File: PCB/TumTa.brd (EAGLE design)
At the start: 100 x 80 mm, 20 parts

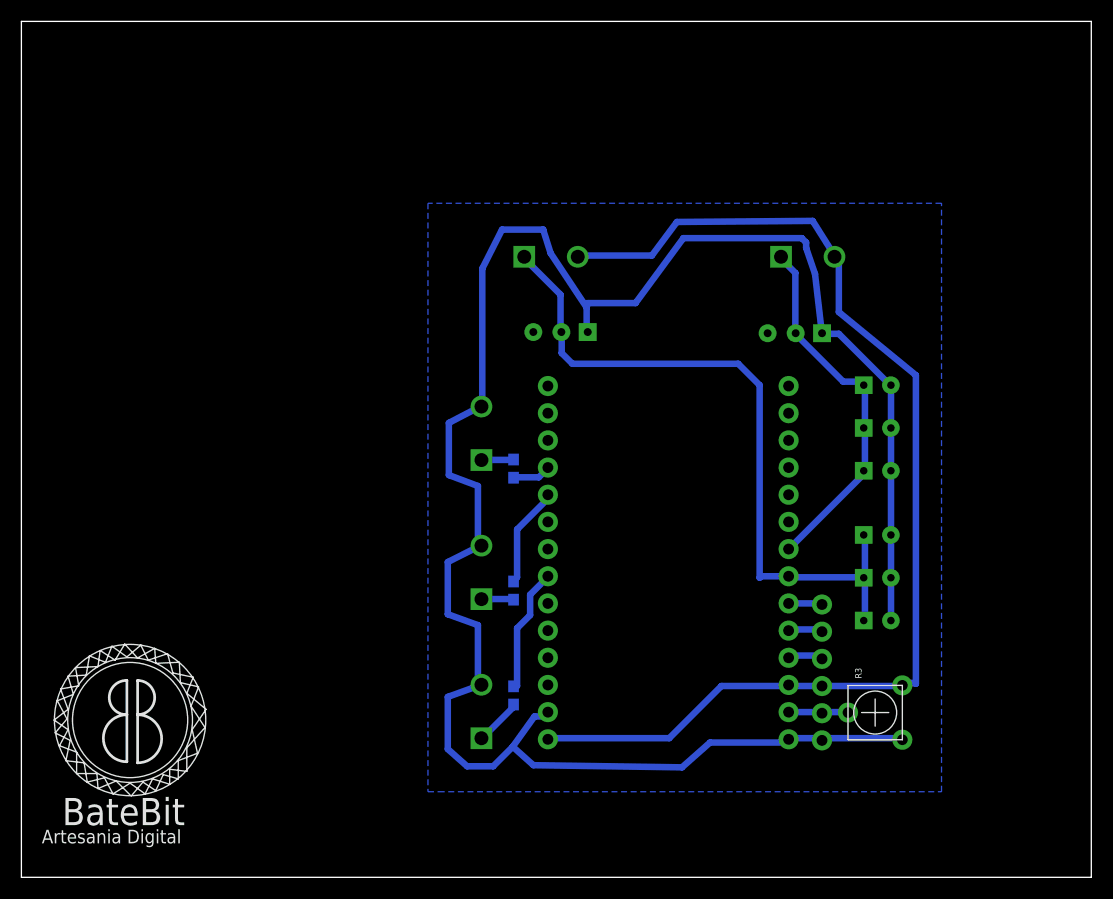
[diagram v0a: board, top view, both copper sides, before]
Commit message: v0_2_8
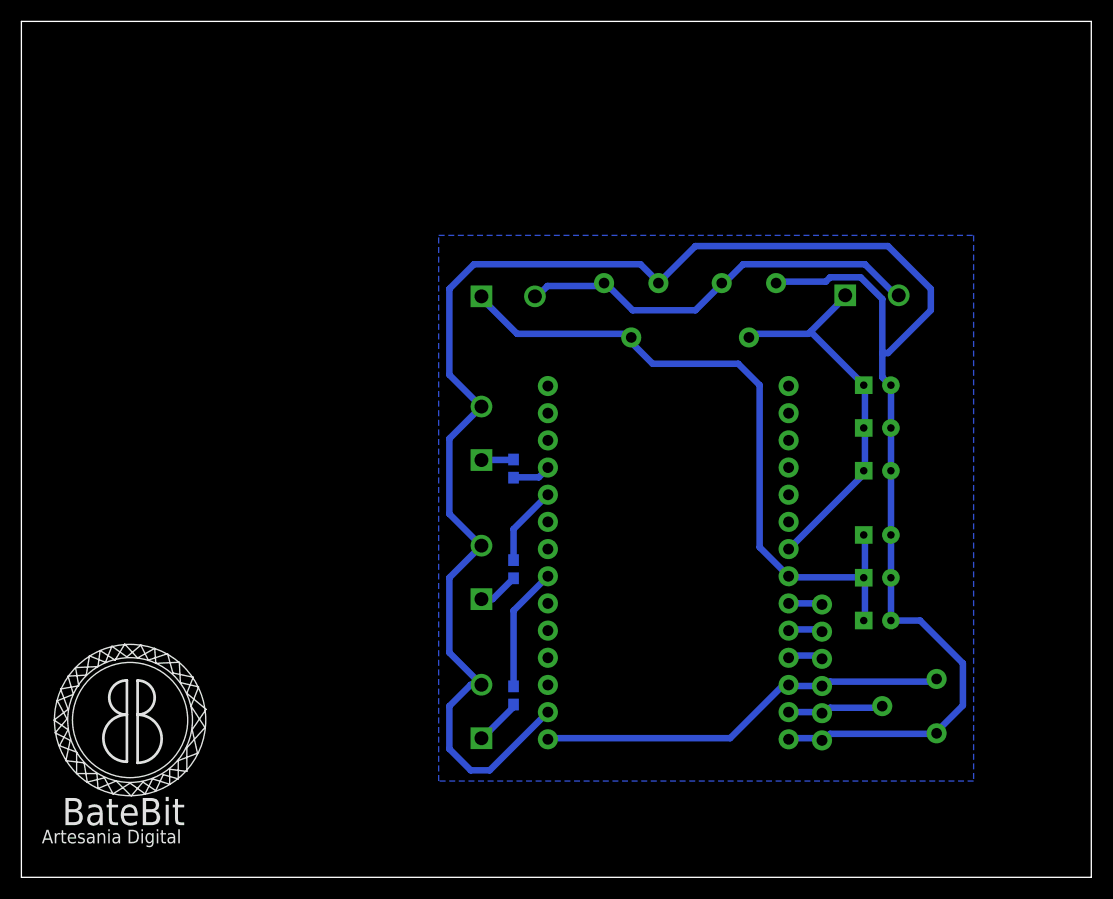
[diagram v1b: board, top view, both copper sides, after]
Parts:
- removed CAL_TA, CAL_TUM: TRIMPOT_MULTIVOLTAS, SparkFun-Electromechanical:TRIMPOT_MULTIVOLTAS
- removed R3: (no value), SparkFun-Electromechanical:TRIM_POT_PTH
- added AREF, TA_CALIB, TUM_CALIB: (no value), SparkFun-Electromechanical:TRIM_POT_BR
- moved TA 7.00 mm to (77.0, 54.4)
- moved TUM 5.45 mm to (43.0, 54.3)
- moved R1 2.00 mm to (46.0, 28.8)
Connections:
- new net 3.3V: TA.2, TA_CALIB.3, TUM.2, TUM_CALIB.3
- net 3V3: now also AREF.3; no longer R3.3, TA.2, TUM.2
- net A0: now also TUM_CALIB.2; no longer CAL_TUM.2
- net A1: now also TA_CALIB.2; no longer CAL_TA.2
- net AREF: now also AREF.2; no longer R3.2
- net GND: now also AREF.1, TA_CALIB.1, TUM_CALIB.1; no longer CAL_TA.1, CAL_TUM.1, R3.1
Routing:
- net 3V3: track 107.8 -> 39.0 mm
- net 3.3V: track 0.00 -> 38.9 mm
- net GND: track 188.7 -> 193.7 mm
- net AREF: track 5.65 -> 9.02 mm
- net A0: track 66.1 -> 64.1 mm
- net D9: track 9.41 -> 7.44 mm
- net A1: track 34.7 -> 36.2 mm
- net N$3: track 3.02 -> 3.81 mm
